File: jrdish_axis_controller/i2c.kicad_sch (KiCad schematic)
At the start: 16 parts, among them U2 ISO1540QDRQ1, U8 LTC4311ISC6#TRPBF, U9 LM75BIMX-5/NOPB

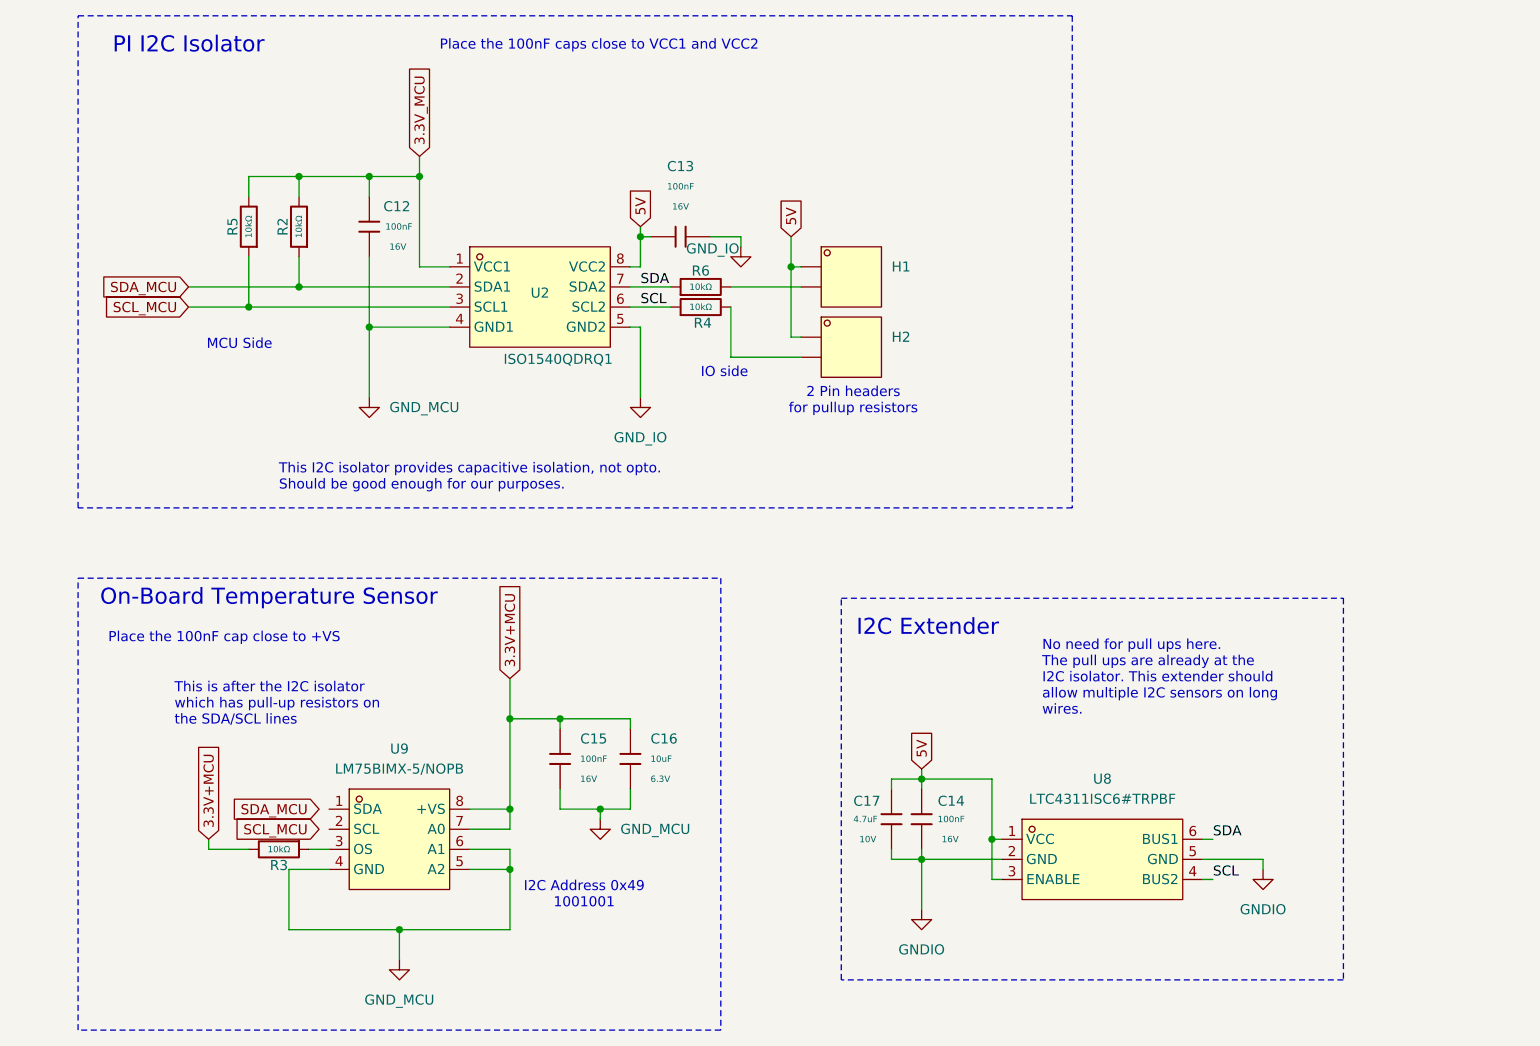
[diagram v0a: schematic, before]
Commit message: Updates
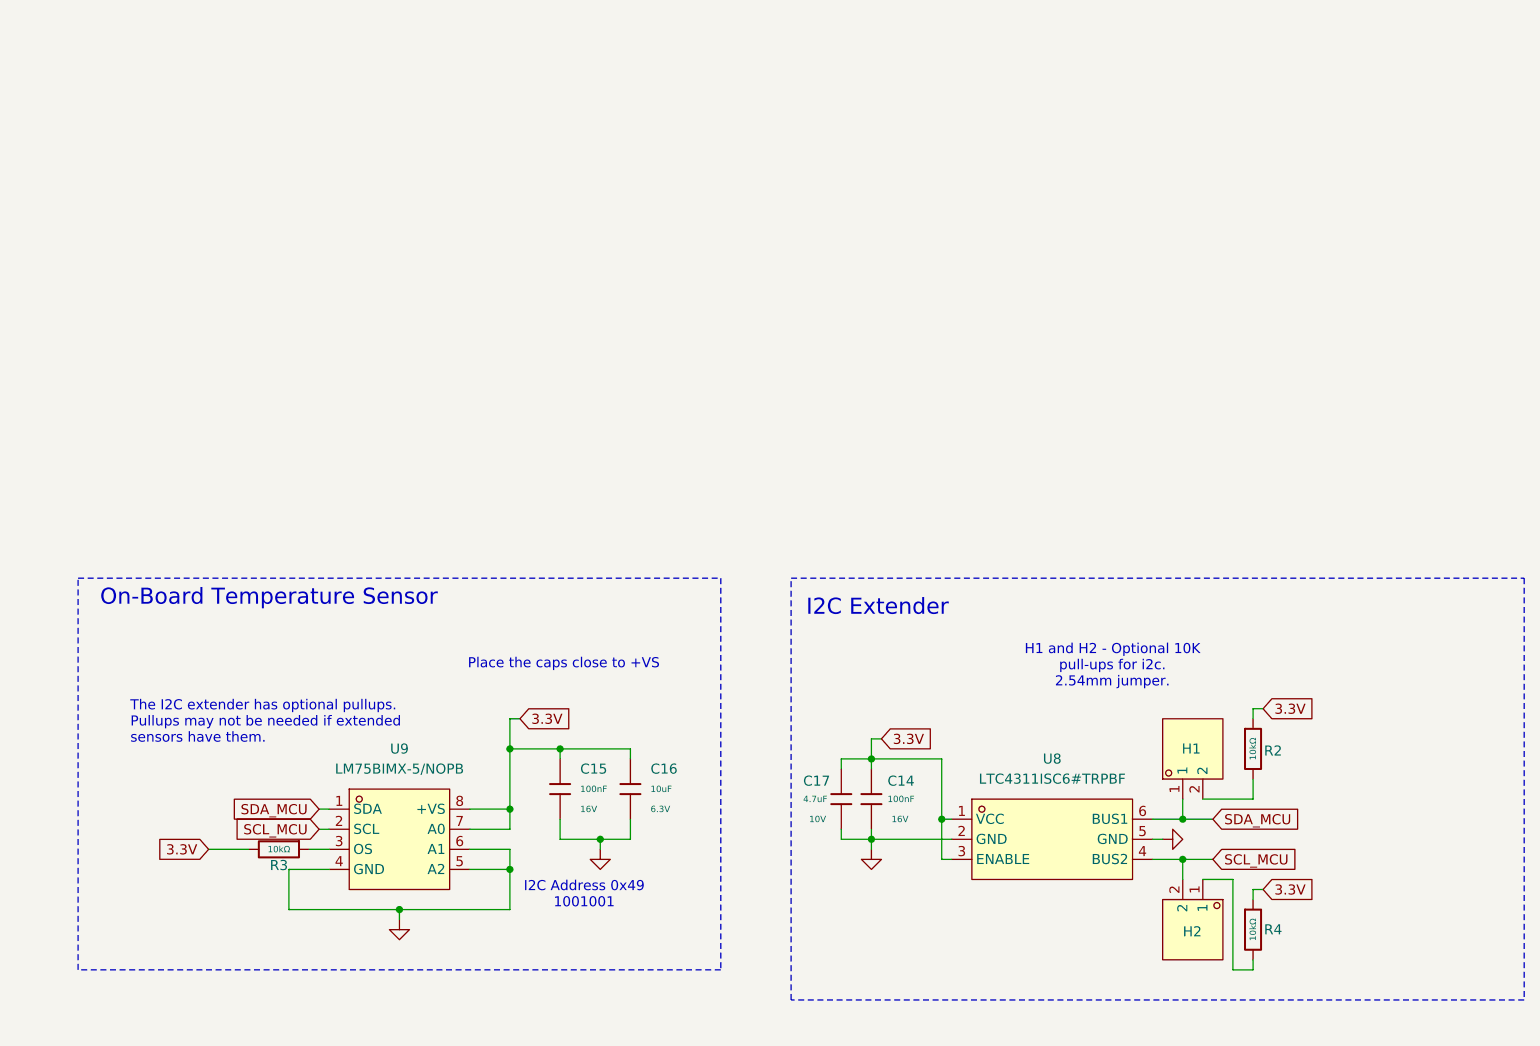
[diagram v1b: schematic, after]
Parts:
- removed C12, C13: 100nF, PCM_JLCPCB:C_0402, symbol PCM_JLCPCB-Capacitors:0402,100nF
- removed R5, R6: 10kΩ, PCM_JLCPCB:R_0402, symbol PCM_JLCPCB-Resistors:0402,10kΩ
- removed U2: ISO1540QDRQ1, MyParts:SOIC-8_L4.9-W3.9-P1.27-LS6.0-BL, symbol MyParts:ISO1540QDRQ1
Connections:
- net 3.3V_MCU is gone; now on an unnamed net: R2.2
- net GND_MCU is gone; now on net GND: C15.2, C16.2, U9.4 (GND), U9.5 (A2), U9.6 (A1)
- net SDA is gone; now on net SDA_MCU: U8.6 (BUS1)
- net SCL_MCU: now also H2.2, U8.4 (BUS2), U9.2 (SCL)
- net SDA_MCU: now also H1.1, U9.1 (SDA); no longer R2.1
- net at R4.2: now also H2.1; no longer H2.2
- net 3.3V+MCU renamed 3.3V
- net 3.3V: now also C14.1, C17.1, R2.1, R4.1, U8.1 (VCC), U8.3 (ENABLE)
- removed net 5V: C14.1, C17.1, H1.1, H2.1, U8.1 (VCC), U8.3 (ENABLE)
- net GNDIO renamed GND
- removed net SCL: R4.1, U8.4 (BUS2)
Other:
- note added: "H1 and H2 - Optional 10K pull-ups for i2c. 2.54mm jumper."
- note added: "Place the caps close to +VS"
- note added: "The I2C extender has optional pullups. Pullups may not be needed if extended sensors have them."
- note removed: "2 Pin headers for pullup resistors"
- note removed: "IO side"
- note removed: "MCU Side"
- note removed: "No need for pull ups here. The pull ups are already at the I2C isolator. This extender should allow multiple I2C sensors on long wires."
- note removed: "PI I2C Isolator"
- note removed: "Place the 100nF cap close to +VS"
- note removed: "Place the 100nF caps close to VCC1 and VCC2"
- note removed: "This I2C isolator provides capacitive isolation, not opto. Should be good enough for our purposes."
- note removed: "This is after the I2C isolator which has pull-up resistors on the SDA/SCL lines"
- moved on the sheet: C14, C15, C16, C17, U8

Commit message: Passes ERC
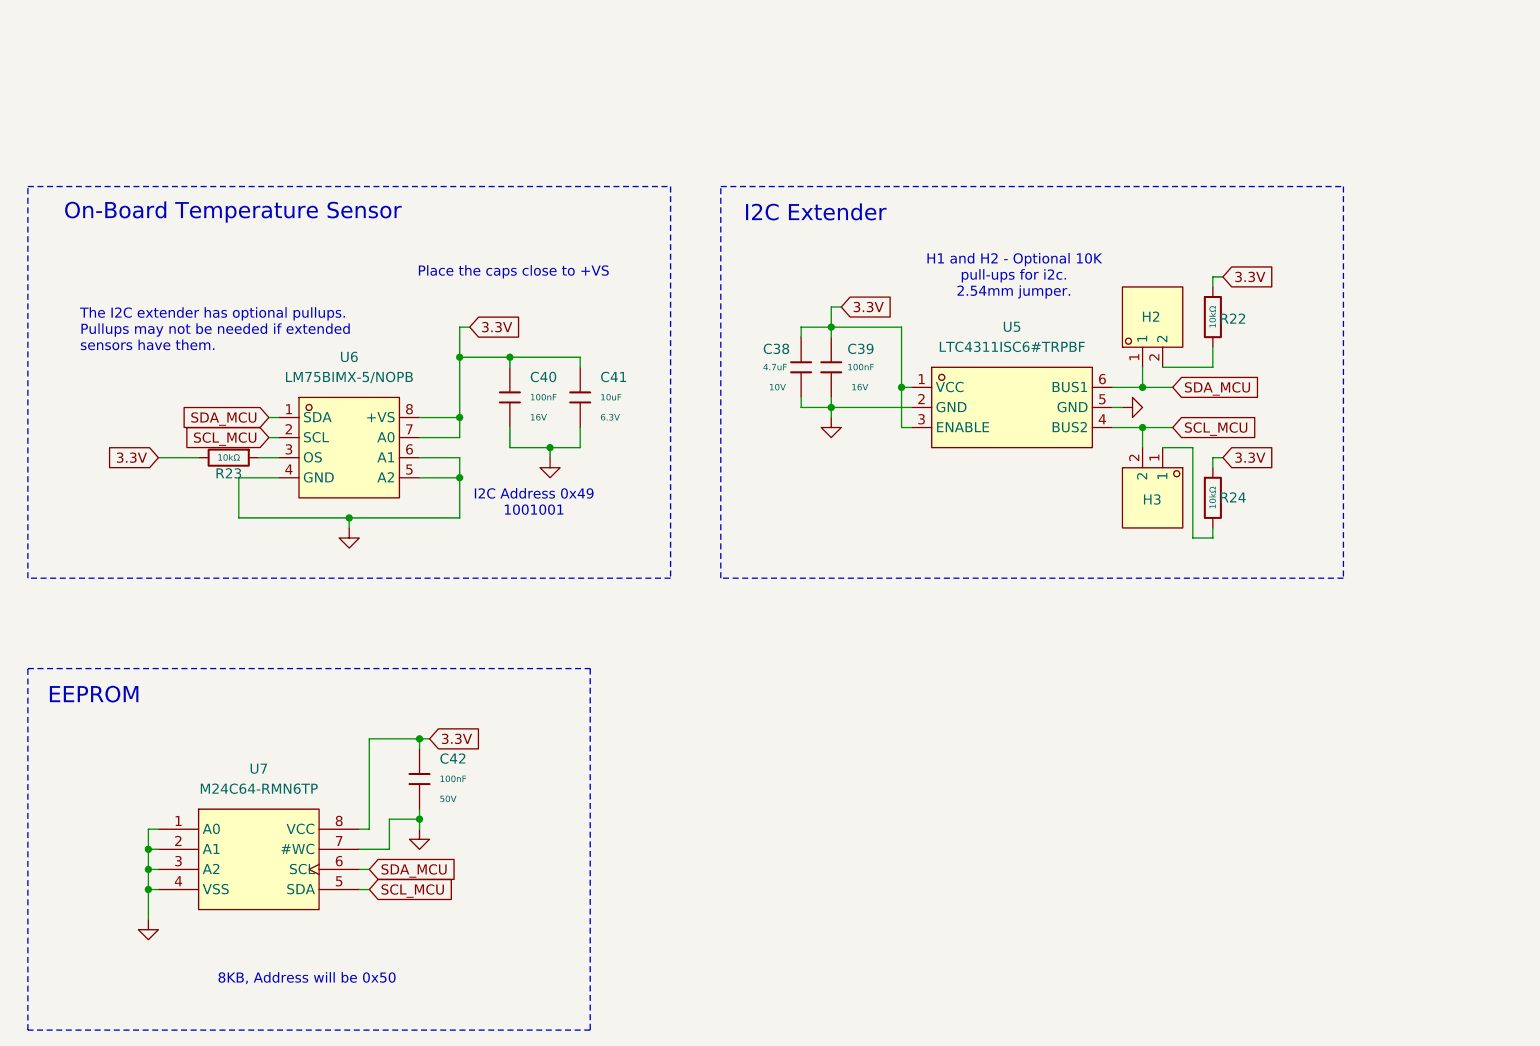
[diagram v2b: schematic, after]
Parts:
- added C42: 100nF, PCM_JLCPCB:C_0402, symbol PCM_JLCPCB-Capacitors:0402,100nF,(2)
- added U7: M24C64-RMN6TP, MyParts:SOIC-8_L5.0-W4.0-P1.27-LS6.0-BL, symbol MyParts:M24C64-RMN6TP
- renumbered C17 to C38, C14 to C39, C15 to C40, C16 to C41, H1 to H2, H2 to H3, R2 to R22, R3 to R23, R4 to R24, U8 to U5, U9 to U6
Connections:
- net 3.3V: now also C42.1, U7.8 (VCC)
- net GND: now also C42.2, U7.1 (A0), U7.2 (A1), U7.3 (A2), U7.4 (VSS), U7.7 (#WC)
- net SCL_MCU: now also U7.5 (SDA)
- net SDA_MCU: now also U7.6 (SCL)
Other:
- note added: "8KB, Address will be 0x50"
- note added: "EEPROM"
- moved on the sheet: C38, C39, C40, C41, H2, H3, R22, R23, R24, U5, U6
